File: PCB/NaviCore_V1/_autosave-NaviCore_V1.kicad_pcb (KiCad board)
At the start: 2 copper layers, 8 parts, among them J1 SBUS_IN, J2 SBUS_OUT, J3 MAESTRO, J4 SERIAL_1, J5 SEREIAL_2, J6 SERIAL_3, J7 Screw_Terminal_01x02, U1 ESP32-S3-DEVKITC-1-N8R2

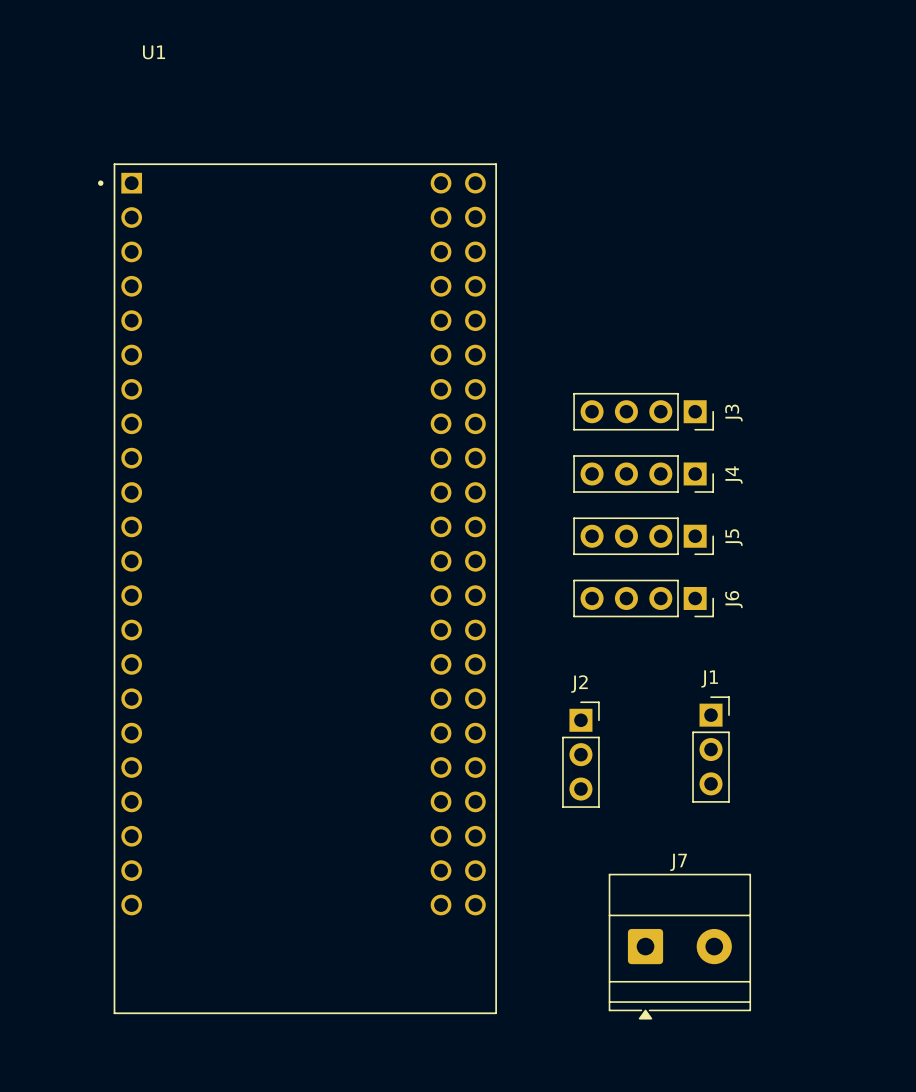
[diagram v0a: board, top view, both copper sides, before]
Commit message: wokring on custom pcb
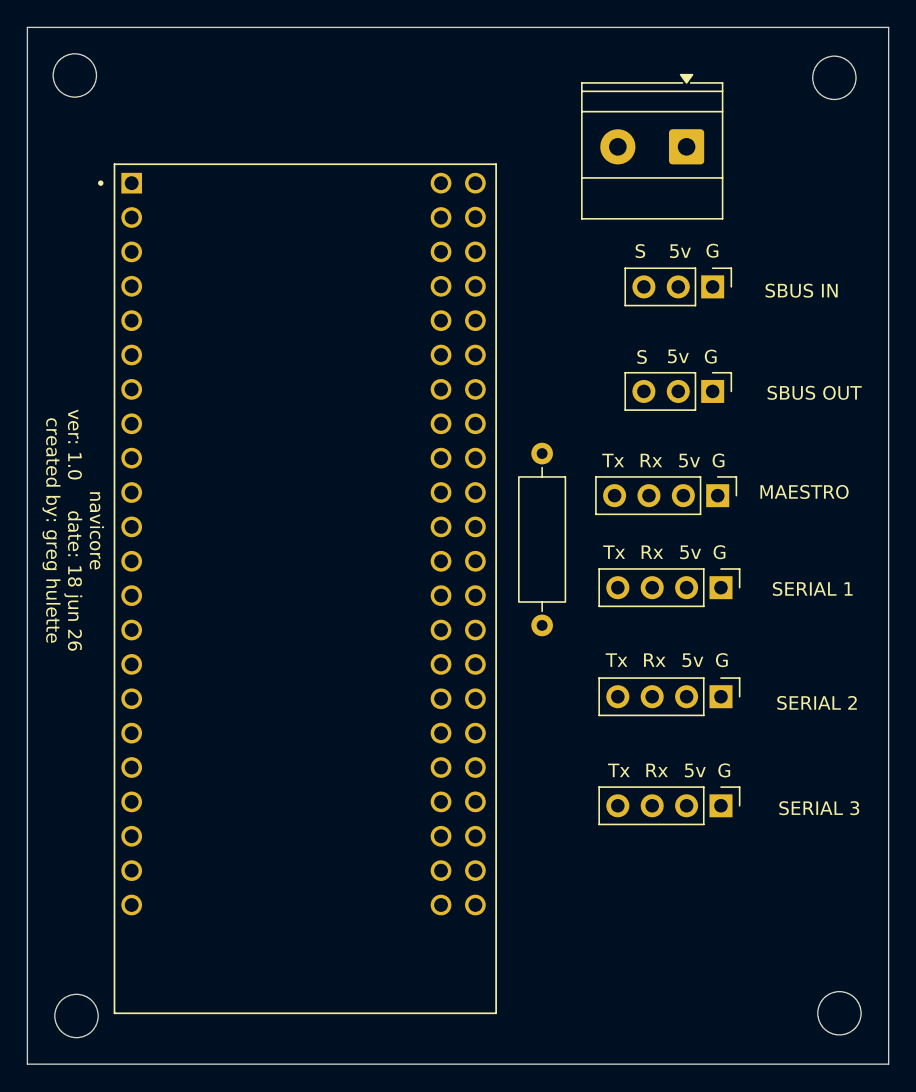
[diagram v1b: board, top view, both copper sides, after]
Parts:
- added H1: MountingHole, MountingHole:MountingHole_3.2mm_M3, F.Cu at (188.3, 53.9)
- added H2: MountingHole, MountingHole:MountingHole_3.2mm_M3, F.Cu at (132.2, 53.7)
- added H3: MountingHole, MountingHole:MountingHole_3.2mm_M3, F.Cu at (188.7, 123.0)
- added H4: MountingHole, MountingHole:MountingHole_3.2mm_M3, F.Cu at (132.3, 123.2)
- added R1: R_Small, Resistor_THT:R_Axial_DIN0309_L9.0mm_D3.2mm_P12.70mm_Horizontal, F.Cu at (166.7, 81.6)
- J1, J2: footprint Connector_PinSocket_2.54mm:PinSocket_1x03_P2.54mm_Vertical -> Connector_PinHeader_2.54mm:PinHeader_1x03_P2.54mm_Vertical
- J3, J4, J5, J6: footprint Connector_PinSocket_2.54mm:PinSocket_1x04_P2.54mm_Vertical -> Connector_PinHeader_2.54mm:PinHeader_1x04_P2.54mm_Vertical
- moved J7 59.2 mm to (177.4, 59.0), turned to 180 degrees
- moved J1 31.6 mm to (179.3, 69.3), turned to -90 degrees
- moved J2 26.2 mm to (179.3, 77.0), turned to -90 degrees
- moved J6 15.4 mm to (179.9, 107.7)
- moved J5 12.0 mm to (179.9, 99.6)
- moved J4 8.61 mm to (179.9, 91.5)
- moved J3 6.42 mm to (179.7, 84.8)
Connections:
- net Net-(U1-3V3-PadJ1_1) renamed 3.3V
- J1 pad 1: unconnected-(J1-Pin_1-Pad1) -> GND
- J1 pad 2: unconnected-(J1-Pin_2-Pad2) -> 5V
- J1 pad 3: unconnected-(J1-Pin_3-Pad3) -> SBUS_IN
- J2 pad 1: unconnected-(J2-Pin_1-Pad1) -> GND
- J2 pad 2: unconnected-(J2-Pin_2-Pad2) -> 5V
- J2 pad 3: unconnected-(J2-Pin_3-Pad3) -> SBUS_OUT
- J3 pad 1: unconnected-(J3-Pin_1-Pad1) -> GND
- J3 pad 2: unconnected-(J3-Pin_2-Pad2) -> 5V
- J3 pad 3: unconnected-(J3-Pin_3-Pad3) -> MAESTRO_RX
- J3 pad 4: unconnected-(J3-Pin_4-Pad4) -> MAESTRO_TX
- J4 pad 1: unconnected-(J4-Pin_1-Pad1) -> GND
- J4 pad 2: unconnected-(J4-Pin_2-Pad2) -> 5V
- J4 pad 3: unconnected-(J4-Pin_3-Pad3) -> SERIAL_1_RX
- J4 pad 4: unconnected-(J4-Pin_4-Pad4) -> SERIAL_1_TX
- J5 pad 1: unconnected-(J5-Pin_1-Pad1) -> GND
- J5 pad 2: unconnected-(J5-Pin_2-Pad2) -> 5V
- J5 pad 3: unconnected-(J5-Pin_3-Pad3) -> SERIAL_2_RX
- J5 pad 4: unconnected-(J5-Pin_4-Pad4) -> SERIAL_2_TX
- J6 pad 1: unconnected-(J6-Pin_1-Pad1) -> GND
- J6 pad 2: unconnected-(J6-Pin_2-Pad2) -> 5V
- J6 pad 3: unconnected-(J6-Pin_3-Pad3) -> SERIAL_3_RX
- J6 pad 4: unconnected-(J6-Pin_4-Pad4) -> SERIAL_3_TX
- J7 pad 1: unconnected-(J7-Pin_1-Pad1) -> GND
- J7 pad 2: unconnected-(J7-Pin_2-Pad2) -> 5V
- U1 pad J1_12: unconnected-(U1-GPIO8-PadJ1_12) -> SERIAL_1_TX
- U1 pad J1_15: unconnected-(U1-GPIO9-PadJ1_15) -> SERIAL_1_RX
- U1 pad J1_16: unconnected-(U1-GPIO10-PadJ1_16) -> SERIAL_2_TX
- U1 pad J1_21: unconnected-(U1-5V0-PadJ1_21) -> 5V
- U1 pad J1_22: Net-(U1-GND-PadJ1_22) -> GND
- U1 pad J1_4: unconnected-(U1-GPIO4-PadJ1_4) -> SBUS_IN
- U1 pad J1_5: unconnected-(U1-GPIO5-PadJ1_5) -> SBUS_OUT
- U1 pad J1_6: unconnected-(U1-GPIO6-PadJ1_6) -> MAESTRO_TX
- U1 pad J1_7: unconnected-(U1-GPIO7-PadJ1_7) -> MAESTRO_RX
- U1 pad J3_1: Net-(U1-GND-PadJ1_22) -> GND
- U1 pad J3_10: unconnected-(U1-GPIO38-PadJ3_10) -> SERIAL_3_TX
- U1 pad J3_14: unconnected-(U1-GPIO0-PadJ3_14) -> Net-(U1-GPIO0)
- U1 pad J3_17: unconnected-(U1-GPIO47-PadJ3_17) -> SERIAL_3_RX
- U1 pad J3_18: unconnected-(U1-GPIO21-PadJ3_18) -> SERIAL_2_RX
- U1 pad J3_21: Net-(U1-GND-PadJ1_22) -> GND
- U1 pad J3_22: Net-(U1-GND-PadJ1_22) -> GND
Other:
- board outline added: 63.6 x 76.6 mm
- board text added: "5v"
- board text added: "G"
- board text added: "MAESTRO"
- board text added: "Rx"
- board text added: "S"
- board text added: "SBUS IN"
- board text added: "SBUS OUT"
- board text added: "SERIAL 1"
- board text added: "SERIAL 2"
- board text added: "SERIAL 3"
- board text added: "Tx"
- board text added: "navicore ver: 1.0 date: 18 jun 26 created by: greg hulette"
